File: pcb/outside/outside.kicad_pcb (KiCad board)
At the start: 2 copper layers, 72 parts, among them J1 USB_C_Receptacle_USB2.0_16P, J2 RJ12, J3 Conn_01x08, J4 Conn_01x04, Q1 BSS138, SW1 RST, SW2 PRG, U1 ESP32-C6-MINI-1, U2 MFRC52201HN1,157, U3 USBLC6-2SC6, U4 AMS1117-3.3, U5 USBLC6-2SC6, Y1 27.12MHz

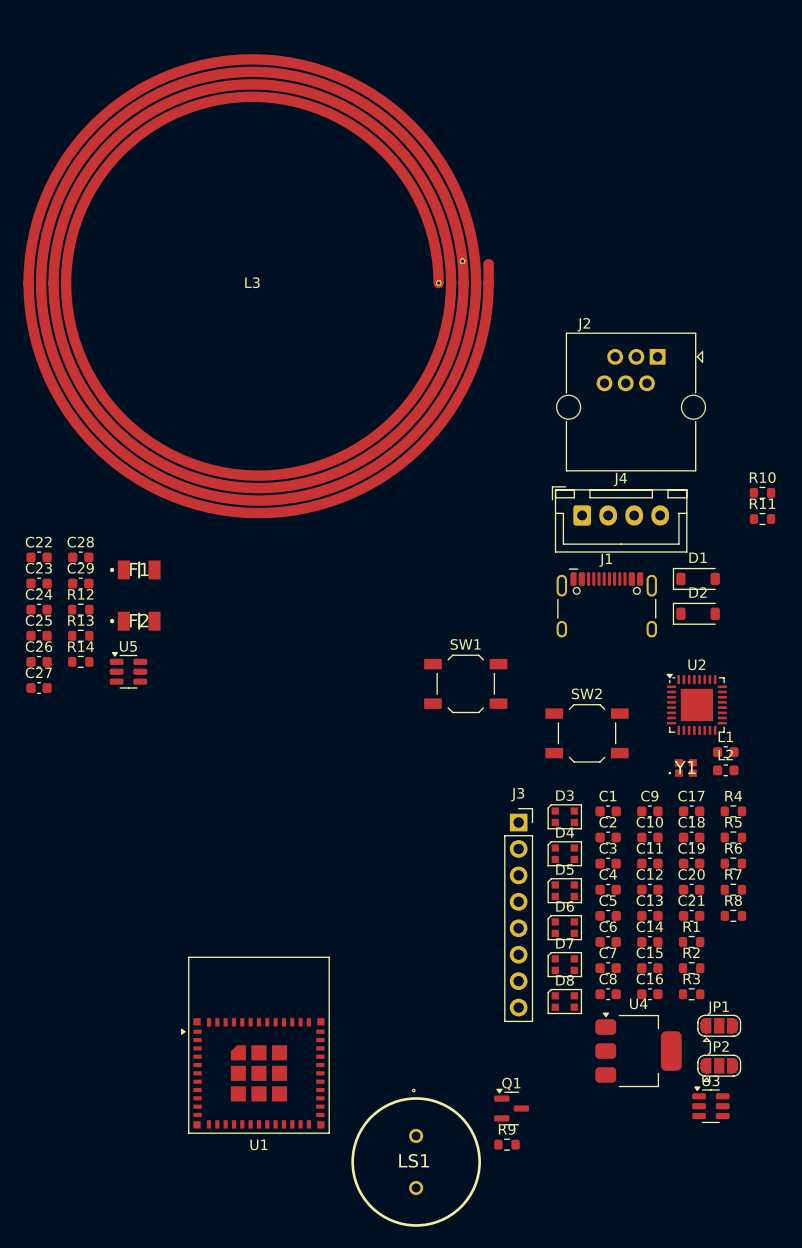
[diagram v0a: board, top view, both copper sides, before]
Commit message: feat: initial PCB
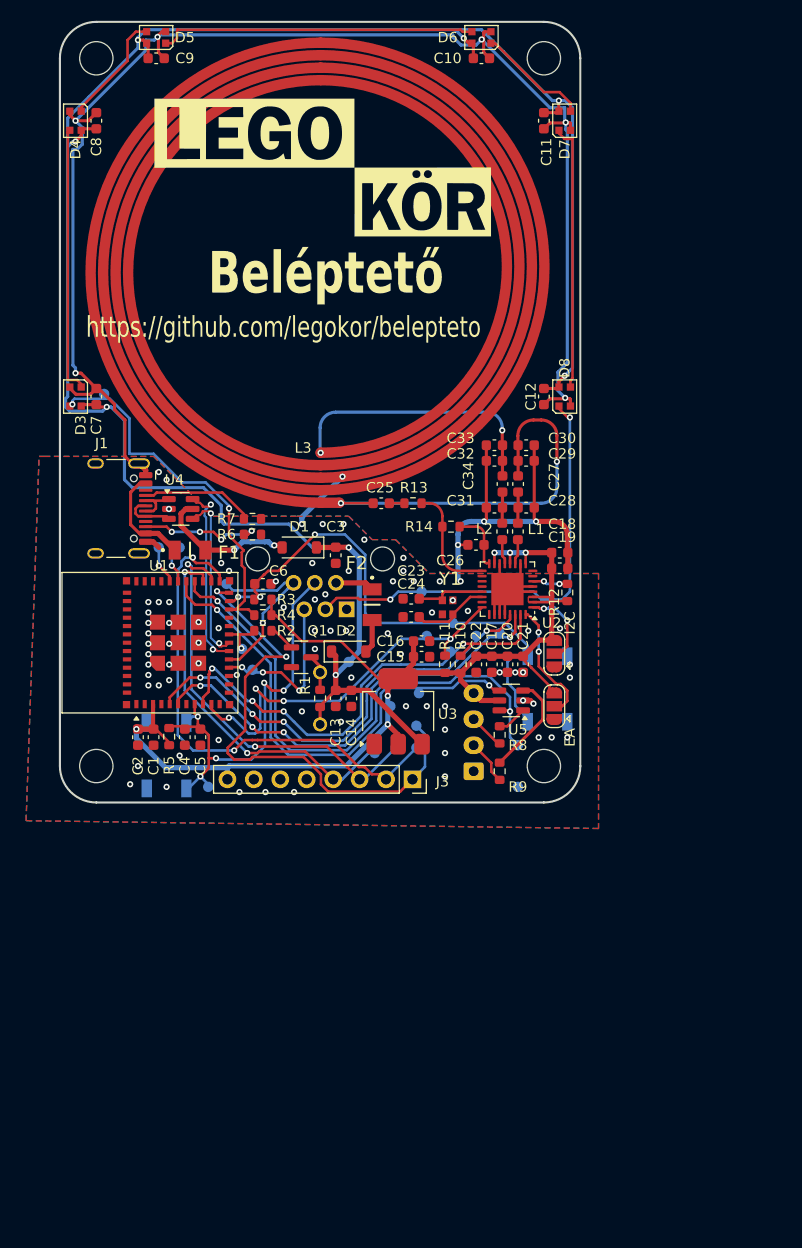
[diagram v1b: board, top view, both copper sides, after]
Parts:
- removed the C22 at (98.0, 76.5)
- removed the C25 at (98.0, 84.0)
- removed the C27 at (98.0, 89.0)
- removed the C28 at (102.0, 76.5)
- removed the C29 at (102.0, 79.0)
- removed the R12 at (102.0, 81.5)
- removed the R13 at (102.0, 84.0)
- removed the R14 at (102.0, 86.5)
- added C10: 100n, Capacitor_SMD:C_0603_1608Metric, F.Cu at (140.5, 28.5)
- added C13: 10u, Capacitor_SMD:C_0603_1608Metric, F.Cu at (126.5, 90.0)
- added C14: 100n, Capacitor_SMD:C_0603_1608Metric, F.Cu at (128.0, 90.0)
- added C15: 100n, Capacitor_SMD:C_0603_1608Metric, F.Cu at (134.8, 86.0)
- added C16: 10u, Capacitor_SMD:C_0603_1608Metric, F.Cu at (134.8, 84.5)
- added C18: 100n, Capacitor_SMD:C_0603_1608Metric, F.Cu at (148.0, 76.0)
- added C19: 100n, Capacitor_SMD:C_0603_1608Metric, F.Cu at (148.0, 77.5)
- added C20: 100n, Capacitor_SMD:C_0603_1608Metric, F.Cu at (143.0, 86.7)
- added C21: 100n, Capacitor_SMD:C_0603_1608Metric, F.Cu at (144.5, 86.7)
- added C9: 100n, Capacitor_SMD:C_0603_1608Metric, F.Cu at (109.2, 28.5)
- added G***: LOGO, belepteto:LEGO, F.Cu at (125.2, 39.0)
- added H1: MountingHole, MountingHole:MountingHole_3.2mm_M3, F.Cu at (103.5, 28.5)
- added H2: MountingHole, MountingHole:MountingHole_3.2mm_M3, F.Cu at (103.5, 96.5)
- added H3: MountingHole, MountingHole:MountingHole_3.2mm_M3, F.Cu at (146.5, 28.5)
- added H4: MountingHole, MountingHole:MountingHole_3.2mm_M3, F.Cu at (146.5, 96.5)
- added R6: 5k1, Resistor_SMD:R_0603_1608Metric, F.Cu at (118.5, 74.2)
- added R7: 5k1, Resistor_SMD:R_0603_1608Metric, F.Cu at (118.5, 72.8)
- added R8: 22, Resistor_SMD:R_0603_1608Metric, F.Cu at (142.2, 93.5)
- added TP1: BUZZER, TestPoint:TestPoint_Pad_D1.0mm, B.Cu at (117.5, 85.2)
- added TP10: OUT2, TestPoint:TestPoint_Pad_D1.0mm, B.Cu at (116.0, 79.0)
- added TP11: OUT1, TestPoint:TestPoint_Pad_D1.0mm, B.Cu at (118.5, 87.2)
- added TP12: EXT_MISO, TestPoint:TestPoint_Pad_D1.0mm, B.Cu at (130.2, 95.2)
- added TP13: EXT_MOSI, TestPoint:TestPoint_Pad_D1.0mm, B.Cu at (132.2, 94.8)
- added TP14: EXT_SCLK, TestPoint:TestPoint_Pad_D1.0mm, B.Cu at (134.2, 94.8)
- added TP15: EXT_CS, TestPoint:TestPoint_Pad_D1.0mm, B.Cu at (134.2, 92.6)
- added TP16: LED_IN, TestPoint:TestPoint_Pad_D1.0mm, B.Cu at (104.2, 60.8)
- added TP17: LED_OUT, TestPoint:TestPoint_Pad_D1.0mm, B.Cu at (134.8, 79.8)
- added TP18: FPRINT_RX, TestPoint:TestPoint_Pad_D1.0mm, B.Cu at (144.0, 94.5)
- added TP19: FPRINT_TX, TestPoint:TestPoint_Pad_D1.0mm, B.Cu at (134.5, 89.5)
- added TP2: ESP_RST, TestPoint:TestPoint_Pad_D1.0mm, B.Cu at (114.2, 98.5)
- added TP20: +5V, TestPoint:TestPoint_Pad_D1.0mm, B.Cu at (127.8, 86.5)
- added TP21: +3V3, TestPoint:TestPoint_Pad_D1.0mm, B.Cu at (131.8, 90.8)
- added TP22: GND, TestPoint:TestPoint_Pad_D1.0mm, B.Cu at (144.0, 98.5)
- added TP3: ESP_TX, TestPoint:TestPoint_Pad_D1.0mm, B.Cu at (109.5, 75.5)
- added TP4: ESP_RX, TestPoint:TestPoint_Pad_D1.0mm, B.Cu at (111.5, 75.5)
- added TP5: ESP_PRG, TestPoint:TestPoint_Pad_D1.0mm, B.Cu at (137.8, 82.8)
- added TP6: INT_CS, TestPoint:TestPoint_Pad_D1.0mm, B.Cu at (135.2, 84.0)
- added TP7: INT_SCLK, TestPoint:TestPoint_Pad_D1.0mm, B.Cu at (140.0, 84.0)
- added TP8: INT_MISO, TestPoint:TestPoint_Pad_D1.0mm, B.Cu at (137.5, 85.5)
- added TP9: INT_MOSI, TestPoint:TestPoint_Pad_D1.0mm, B.Cu at (142.2, 83.8)
- C1, C6: value 10u -> 100n
- C11, C12: value 15p -> 100n
- C23, C24: value 100n -> 15p
- C3: value 100n -> 10u
- C4: value 10u -> 1u
- C8: value 1u -> 100n
- J2, J4, LS1, SW1, SW2: moved to B.Cu
- R1: value 5k1 -> 1k
- R2: value 5k1 -> 180
- R9: value 1k -> 22
- U3: value USBLC6-2SC6 -> AMS1117-3.3; footprint Package_TO_SOT_SMD:SOT-23-6 -> Package_TO_SOT_SMD:SOT-223-3_TabPin2
- U4: value AMS1117-3.3 -> USBLC6-2SC6; footprint Package_TO_SOT_SMD:SOT-223-3_TabPin2 -> Package_TO_SOT_SMD:SOT-23-6
- moved C8 97.3 mm to (103.5, 34.5), turned to -90 degrees
- moved D5 90.9 mm to (109.2, 26.5), turned to 180 degrees
- moved D6 85.9 mm to (140.5, 26.5), turned to 180 degrees
- moved D4 84.7 mm to (101.5, 34.5), turned to -90 degrees
- moved D7 81.1 mm to (148.5, 34.5), turned to 90 degrees
- moved C7 73.7 mm to (103.5, 61.0), turned to -90 degrees
- moved C11 72.1 mm to (146.5, 34.5), turned to 90 degrees
- moved U4 68.2 mm to (111.6, 71.8)
- moved D3 62.0 mm to (101.5, 61.0), turned to -90 degrees
- moved D8 58.1 mm to (148.5, 61.0), turned to 90 degrees
- moved R3 56.0 mm to (119.5, 80.5), turned to 180 degrees
- moved R5 55.1 mm to (110.5, 93.7), turned to 90 degrees
- moved R2 52.4 mm to (119.5, 83.5)
- moved C34 51.0 mm to (142.5, 69.4), turned to 90 degrees
- moved C25 49.6 mm to (130.9, 71.2), turned to 180 degrees
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- renumbered C10 to C17, C9 to C22, C21 to C25, C15 to C27, C13 to C28, C17 to C29, C19 to C30, C14 to C31, C18 to C32, C20 to C33, C16 to C34, R11 to R10, R10 to R11, R6 to R12, R7 to R13, R8 to R14
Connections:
- net /ESP/CS renamed /CS
- net /ESP/EXT_CS renamed /EXT_CS
- net /ESP/EXT_MISO renamed /EXT_MISO
- net /ESP/EXT_MOSI renamed /EXT_MOSI
- net /ESP/EXT_SCLK renamed /EXT_SCLK
- net /ESP/FPRINT_RX renamed /FPRINT_RX
- net /ESP/FPRINT_TX renamed /FPRINT_TX
- net /ESP/MISO renamed /MISO
- net /ESP/MOSI renamed /MOSI
- net /ESP/SCLK renamed /SCLK
- net Net-(U2-NRSTPD) renamed /RFID/RST
- C1 pad 1: +5V -> +3V3
- C11 pad 1: /RFID/OSC2 -> GND
- C11 pad 2: GND -> +5V
- C12 pad 1: /RFID/OSC1 -> GND
- C12 pad 2: GND -> +5V
- C2 pad 1: +5V -> +3V3
- C23 pad 1: GND -> /RFID/OSC2
- C23 pad 2: /RST -> GND
- C24 pad 1: GND -> /RFID/OSC1
- C24 pad 2: +5V -> GND
- C26 pad 1: GND -> /RFID/VMID
- C26 pad 2: +5V -> GND
- C4 pad 1: GND -> /RST
- C4 pad 2: +3V3 -> GND
- C5 pad 2: +3V3 -> /RST
- C6 pad 1: +3V3 -> GND
- C6 pad 2: GND -> /PRG
- C7 pad 1: +3V3 -> GND
- C7 pad 2: GND -> +5V
- C8 pad 1: /RST -> GND
- C8 pad 2: GND -> +5V
- J1 pad A5: Net-(J1-CC1) -> /USB_CC1
- J1 pad A6: Net-(J1-D+-PadA6) -> /USBC+
- J1 pad A7: Net-(J1-D--PadA7) -> /USBC-
- J1 pad B5: Net-(J1-CC2) -> /USB_CC2
- J1 pad B6: Net-(J1-D+-PadA6) -> /USBC+
- J1 pad B7: Net-(J1-D--PadA7) -> /USBC-
- R1 pad 1: Net-(J1-CC1) -> +5V
- R1 pad 2: GND -> Net-(Q1-D)
- R2 pad 1: Net-(J1-CC2) -> /BUZZER
- R2 pad 2: GND -> Net-(Q1-G)
- R3 pad 2: /RST -> /PRG
- R4 pad 2: /ESP/PRG -> /LED_IN
- R5 pad 2: /LED_IN -> /RST
- R9 pad 1: +5V -> Net-(J4-Pin_2)
- R9 pad 2: Net-(Q1-D) -> Net-(R9-Pad2)
- SW2 pad 2: /ESP/PRG -> /PRG
- U1 pad 19: /ESP/BUZZER -> /BUZZER
- U1 pad 23: /ESP/PRG -> /PRG
- U1 pad 30: unconnected-(U1-RXD0-Pad30) -> Net-(U1-RXD0)
- U1 pad 31: unconnected-(U1-TXD0-Pad31) -> Net-(U1-TXD0)
- U2 pad 12: unconnected-(U2-TVDD-Pad12) -> +3V3
- U2 pad 9: unconnected-(U2-SVDD-Pad9) -> +3V3
- U3 pad 1: Net-(J1-D--PadA7) -> GND
- U3 pad 2: GND -> +3V3
- U3 pad 3: Net-(J1-D+-PadA6) -> +5V
- U4 pad 1: GND -> /USBC-
- U4 pad 2: +3V3 -> GND
- U4 pad 3: +5V -> /USBC+
- U5 pad 3: Net-(R14-Pad2) -> Net-(R9-Pad2)
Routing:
- net GND: track 0.00 -> 201.6 mm, vias 0 -> 90
- net +5V: track 0.00 -> 200.0 mm, vias 0 -> 8
- net +3V3: track 0.00 -> 111.6 mm, vias 0 -> 6
- net /FPRINT_RX: track 0.00 -> 53.3 mm, vias 0 -> 2
- net /PRG: track 0.00 -> 51.4 mm, vias 0 -> 3
- net /EXT_CS: track 0.00 -> 49.8 mm, vias 0 -> 2
- net /EXT_SCLK: track 0.00 -> 49.0 mm, vias 0 -> 2
- net /FPRINT_TX: track 0.00 -> 46.9 mm, vias 0 -> 2
- net /MISO: track 0.00 -> 45.5 mm, vias 0 -> 4
- net /MOSI: track 0.00 -> 43.8 mm, vias 0 -> 4
- net /SCLK: track 0.00 -> 43.7 mm, vias 0 -> 4
- net /LED_OUT: track 0.00 -> 43.3 mm, vias 0 -> 2
- net /RST: track 0.00 -> 41.2 mm, vias 0 -> 5
- net /EXT_MOSI: track 0.00 -> 39.9 mm, vias 0 -> 2
- net /CS: track 0.00 -> 38.3 mm, vias 0 -> 4
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- added copper zone on F.Cu, net +3V3
- added copper zone on B.Cu, net GND
- added copper zone on F.Cu, net GND
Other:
- board outline added: 50 x 75 mm
- board text added: "Beléptető"
- board text added: "https://github.com/legokor/belepteto"
